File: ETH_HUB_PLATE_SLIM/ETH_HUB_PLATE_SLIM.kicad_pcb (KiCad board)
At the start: 2 copper layers, 60.5 x 54.4 mm, 6 parts

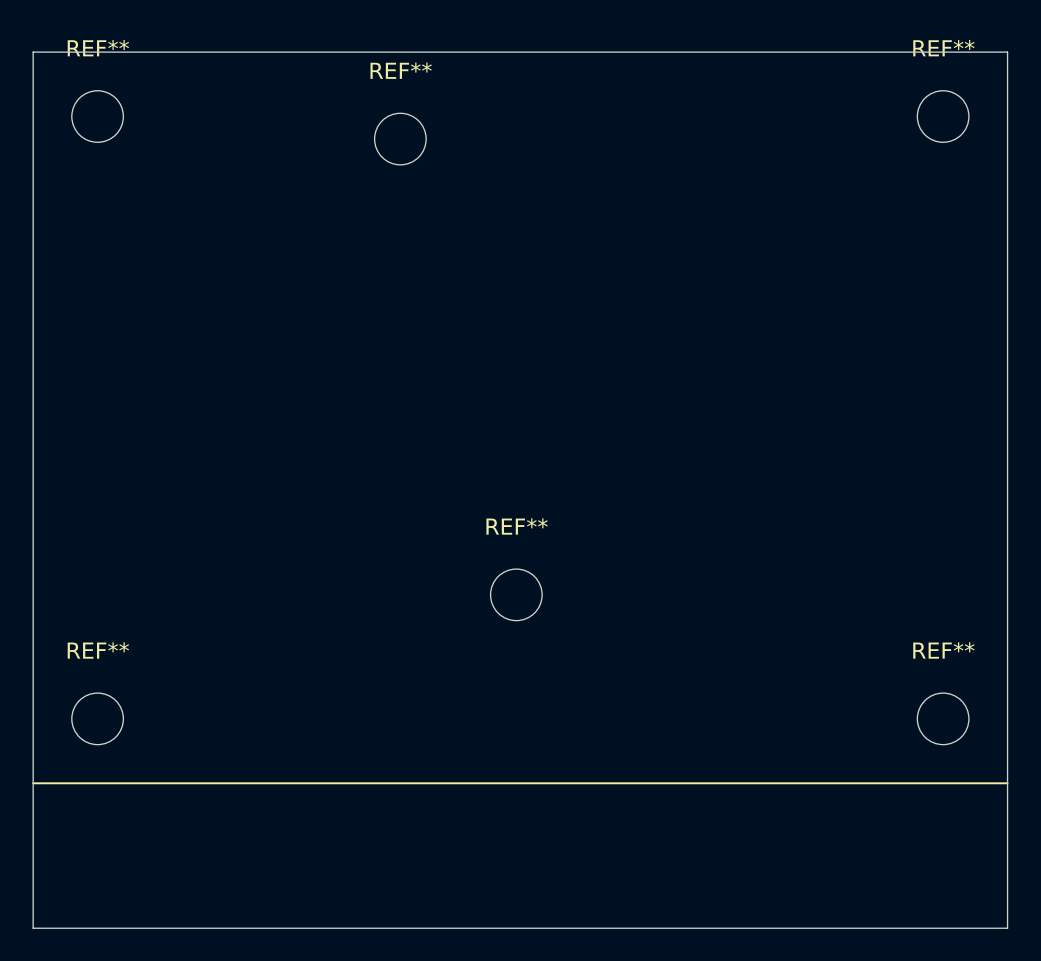
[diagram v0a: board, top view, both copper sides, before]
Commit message: minor adjustments to holes
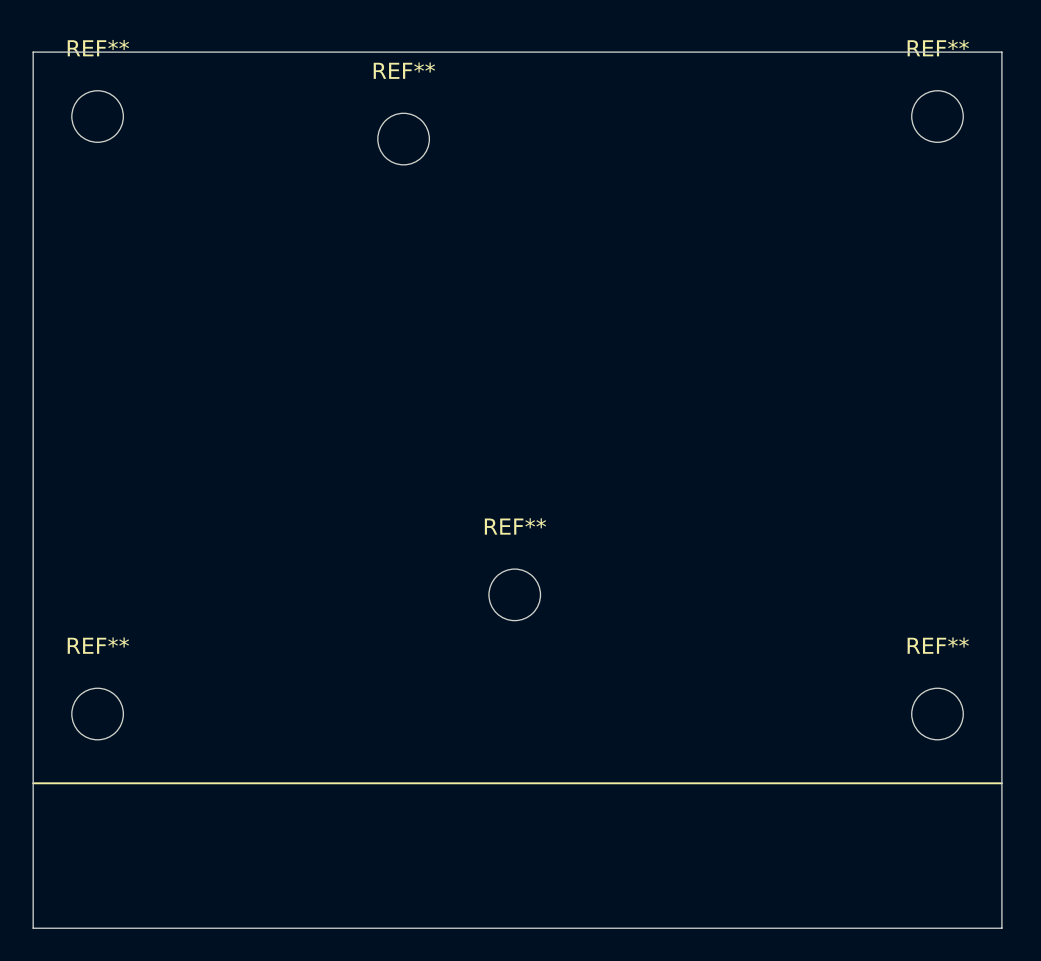
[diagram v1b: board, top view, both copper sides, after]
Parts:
- moved REF** 0.46 mm to (156.2, 141.1)
- moved REF** 0.35 mm to (156.2, 104.0)
- moved REF** 0.30 mm to (104.0, 141.1)
- moved REF** 0.20 mm to (123.0, 105.4)
- moved REF** 0.10 mm to (129.9, 133.7)
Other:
- board size 60.5 x 54.4 mm -> 60.2 x 54.4 mm
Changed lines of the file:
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@@
   )
   (module MountingHole:MountingHole_3.2mm_M3 (layer F.Cu)
-    (at 130 133.7)
+    (at 129.9 133.7)
     (descr "Mounting Hole 3.2mm, no annular, M3")
     (tags "mounting hole 3.2mm no annular m3")
@@
   )
   (module MountingHole:MountingHole_3.2mm_M3 (layer F.Cu)
-    (at 122.8 105.4)
+    (at 123 105.4)
     (descr "Mounting Hole 3.2mm, no annular, M3")
     (tags "mounting hole 3.2mm no annular m3")
@@
   )
   (module MountingHole:MountingHole_3.2mm_M3 (layer F.Cu)
-    (at 156.5 141.4)
+    (at 156.15 141.1)
     (descr "Mounting Hole 3.2mm, no annular, M3")
     (tags "mounting hole 3.2mm no annular m3")
@@
   )
   (module MountingHole:MountingHole_3.2mm_M3 (layer F.Cu)
-    (at 104 141.4)
+    (at 104 141.1)
     (descr "Mounting Hole 3.2mm, no annular, M3")
     (tags "mounting hole 3.2mm no annular m3")
@@
   )
   (module MountingHole:MountingHole_3.2mm_M3 (layer F.Cu)
-    (at 156.5 104)
+    (at 156.15 104)
     (descr "Mounting Hole 3.2mm, no annular, M3")
     (tags "mounting hole 3.2mm no annular m3")
@@
     (pad 1 np_thru_hole circle (at 0 0) (size 3.2 3.2) (drill 3.2) (layers *.Cu *.Mask))
   )
-  (gr_line (start 100 145.4) (end 160.5 145.4) (layer F.SilkS) (width 0.12))
-  (gr_line (start 100 154.4) (end 160.5 154.4) (layer Edge.Cuts) (width 0.05))
-  (gr_line (start 160.5 100) (end 160.5 154.4) (layer Edge.Cuts) (width 0.05))
-  (gr_line (start 100 100) (end 160.5 100) (layer Edge.Cuts) (width 0.05))
+  (gr_line (start 100 145.4) (end 160.15 145.4) (layer F.SilkS) (width 0.12))
+  (gr_line (start 100 154.4) (end 160.15 154.4) (layer Edge.Cuts) (width 0.05))
+  (gr_line (start 160.15 100) (end 160.15 154.4) (layer Edge.Cuts) (width 0.05))
+  (gr_line (start 100 100) (end 160.15 100) (layer Edge.Cuts) (width 0.05))
   (gr_line (start 100 100) (end 100 154.4) (layer Edge.Cuts) (width 0.05))
 )
